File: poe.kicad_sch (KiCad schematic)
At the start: 5 parts, among them J5 Connector_RJ45_Magjack_Abraco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, J6 Connector_RJ45_Magjack_Abraco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, U5 TVS3300DRV

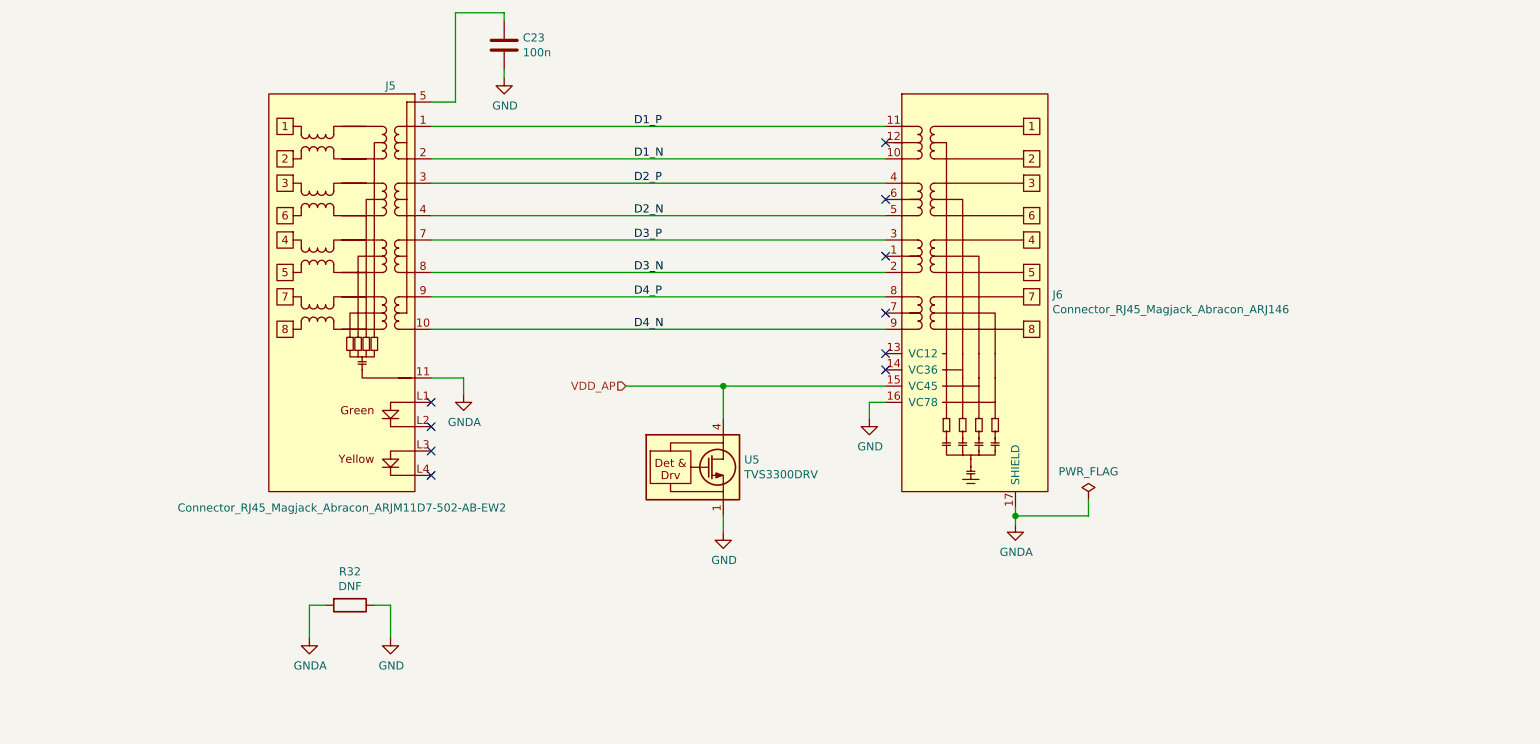
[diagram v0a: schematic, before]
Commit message: Mostly complete, just missing a few tracks and review
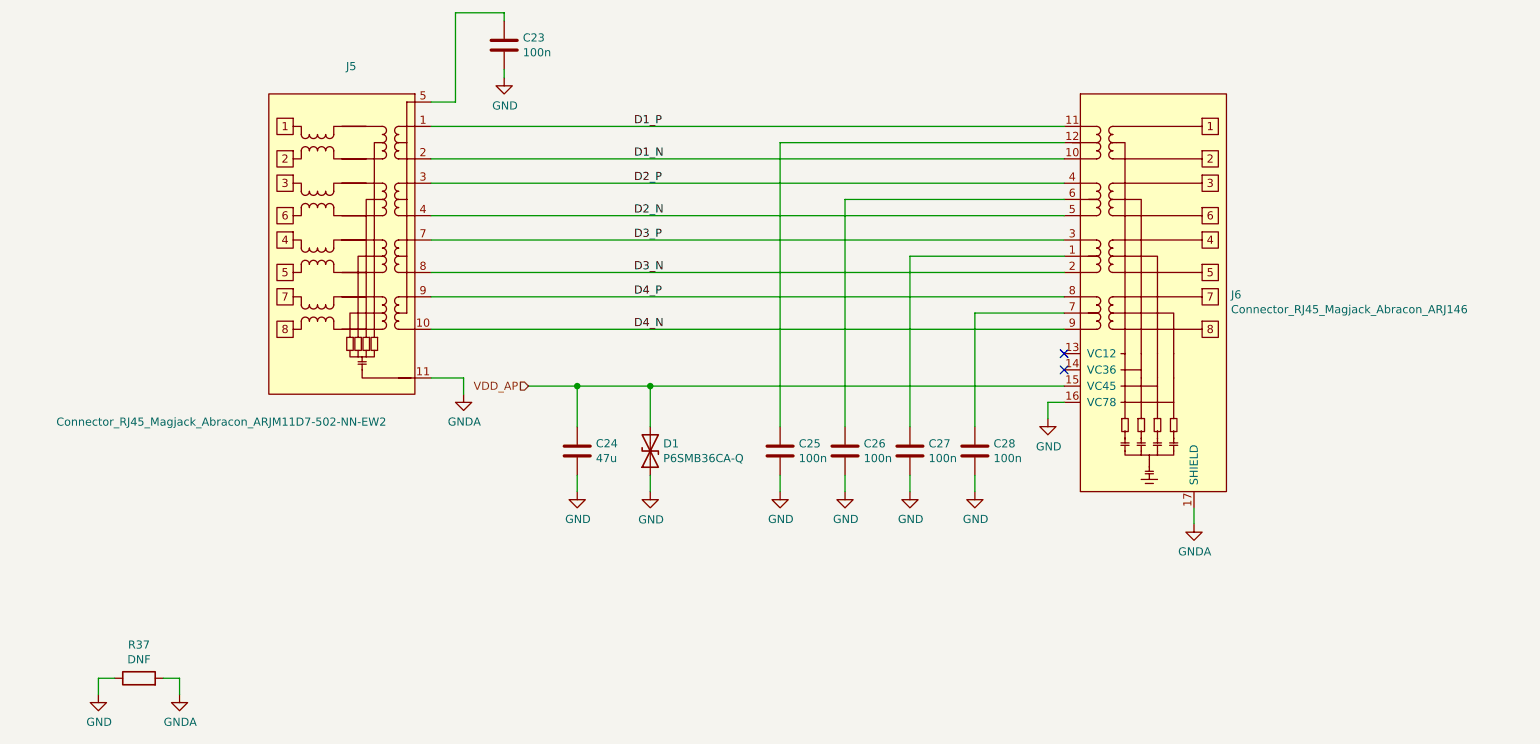
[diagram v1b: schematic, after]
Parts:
- removed J5: Connector_RJ45_Magjack_Abracon_ARJM11D7-502-AB-EW2, Connector_WUT:Connector_RJ45_Magjack_Abracon_ARJM11D7-502-AB-EW2, symbol Connector_WUT:Connector_RJ45_Magjack_Abracon_ARJM11D7-502-AB-EW2
- removed R32: DNF, Resistor_SMD:R_0805_2012Metric, symbol Device:R
- removed U5: TVS3300DRV, Package_SON:WSON-6-1EP_2x2mm_P0.65mm_EP1x1.6mm, symbol Power_Protection:TVS3300DRV
- added C24: 47u, Capacitor_SMD:C_1206_3216Metric, symbol Device:C
- added C25, C26, C27, C28: 100n, Capacitor_SMD:C_0603_1608Metric, symbol Device:C
- added D1: P6SMB36CA-Q, Diode_SMD:D_SMB, symbol Device:D_TVS
- added J5: Connector_RJ45_Magjack_Abracon_ARJM11D7-502-NN-EW2, Connector_WUT:Connector_RJ45_Magjack_Abracon_ARJM11D7-502-NN-EW2, symbol Connector_WUT:Connector_RJ45_Magjack_Abracon_ARJM11D7-502-NN-EW2
- added R37: DNF, Resistor_SMD:R_0603_1608Metric, symbol Device:R
- C23: footprint Capacitor_SMD:C_0402_1005Metric -> Capacitor_SMD:C_0603_1608Metric
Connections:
- net D1_N: now also J5.2
- net D1_P: now also J5.1
- net D2_N: now also J5.4
- net D2_P: now also J5.3
- net D3_N: now also J5.8
- net D3_P: now also J5.7
- net D4_N: now also J5.10
- net D4_P: now also J5.9
- net GND: now also C24.2, C25.2, C26.2, C27.2, C28.2, D1.1 (A1), R37.1
- net GNDA: now also J5.11, R37.2
- net VDD_AP: now also C24.1, D1.2 (A2)
- net at J6.1: now also C27.1
- net at J6.12: now also C25.1
- net at J6.6: now also C26.1
- net at J6.7: now also C28.1
- net at C23.1: now also J5.5, J5.6
- no-connect marks 10 -> 2
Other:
- moved on the sheet: J6
